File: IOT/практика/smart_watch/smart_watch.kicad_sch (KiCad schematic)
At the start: 28 parts, among them J1 Conn_01x02_Pin, J2 USB_C_Receptacle_USB2.0_16P, SW3 SW_Push, U3 KXTJ3-1057, U4 MAX30102, U5 TPS61230DRC, U6 BQ24090DGQ, U7 ESP32-WROOM-32

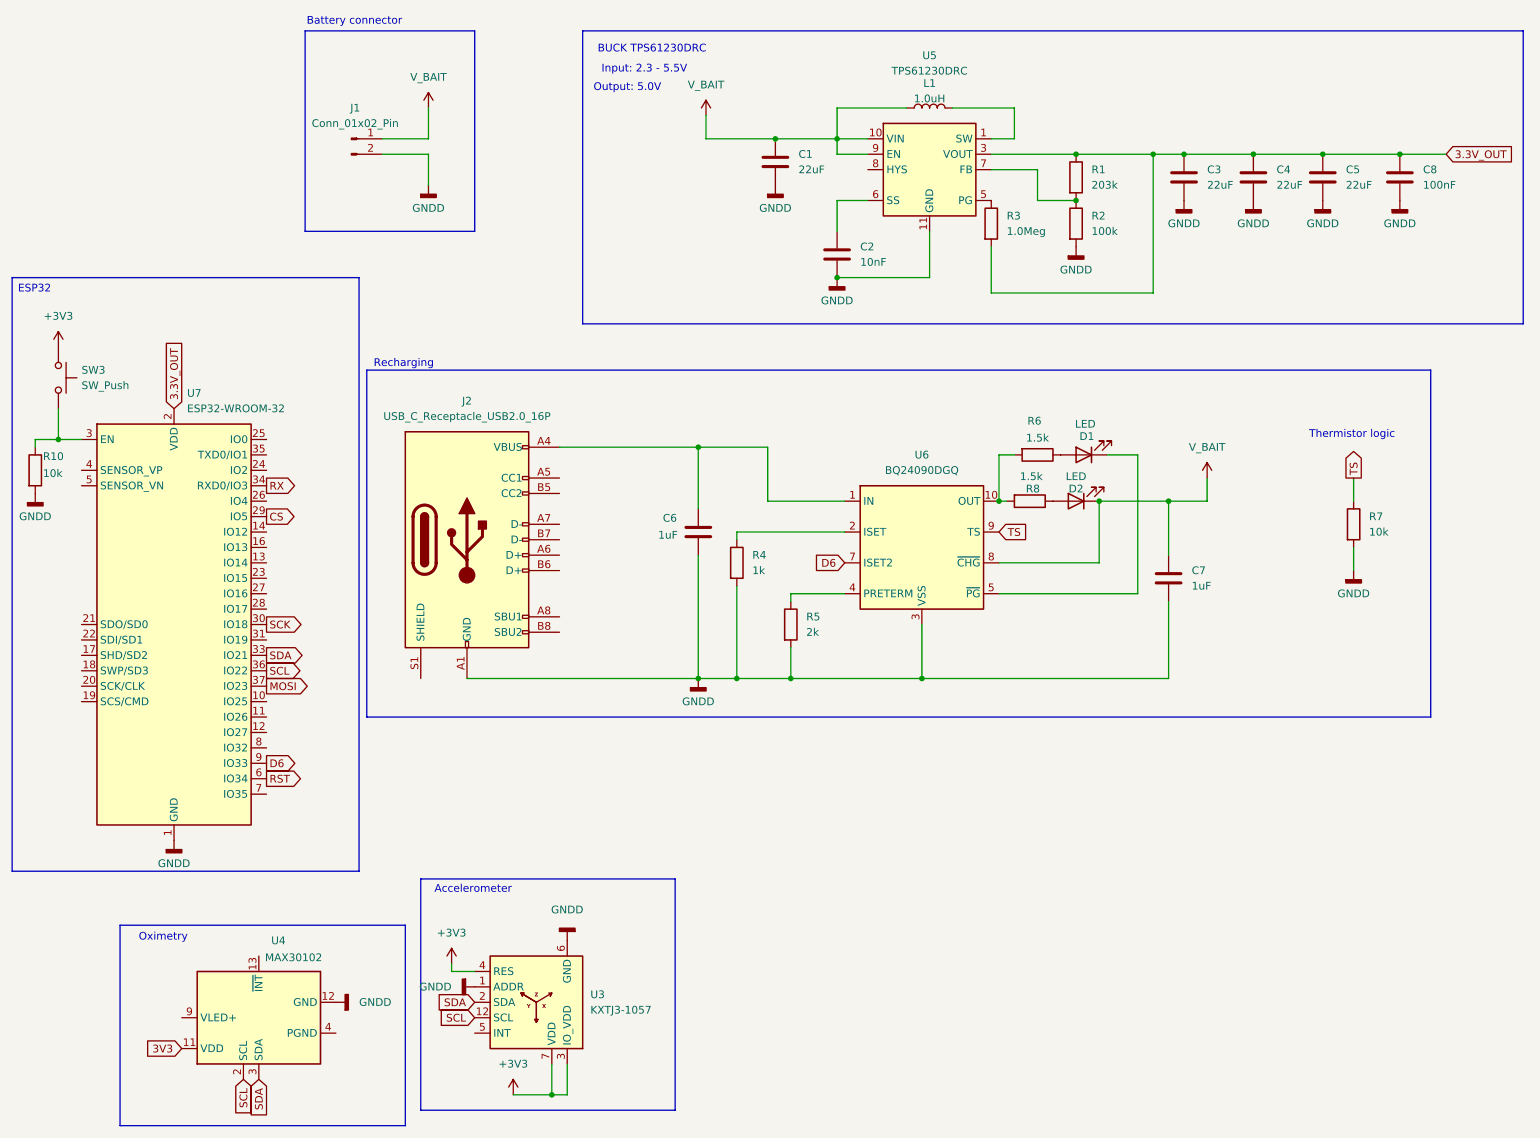
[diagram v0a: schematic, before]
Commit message: feat: adding things
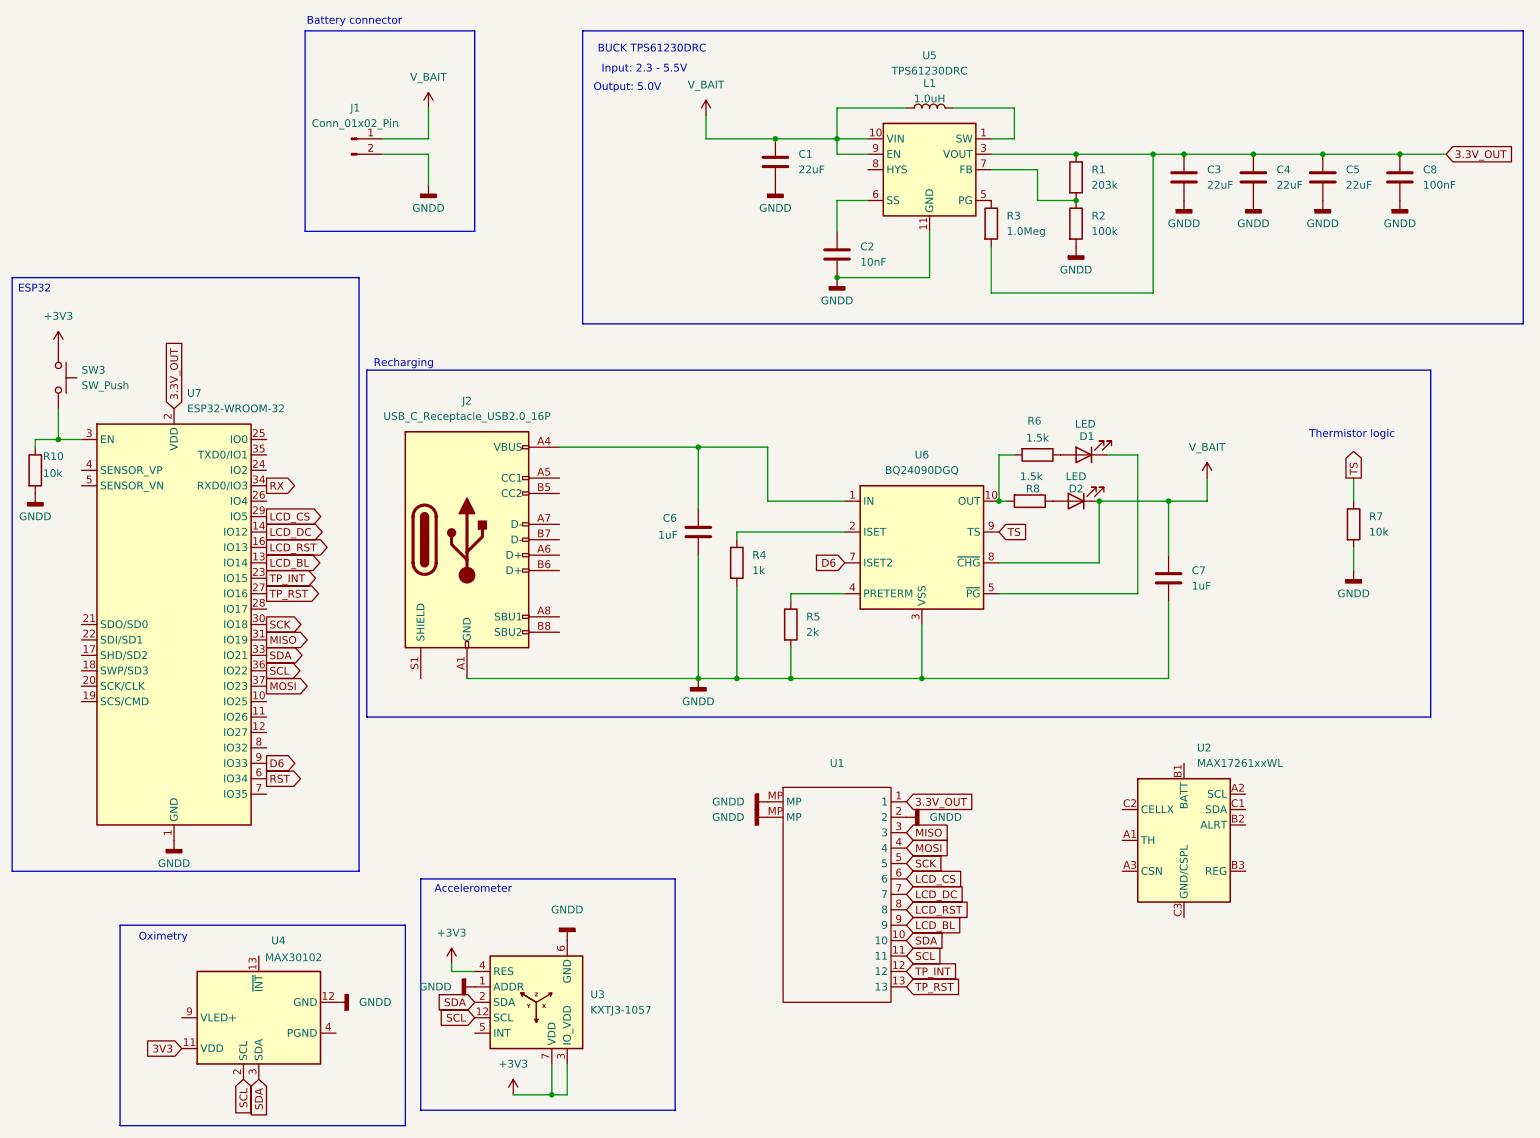
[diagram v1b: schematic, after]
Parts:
- added U1: ~, Connector_FFC:Hirose_FH12-13S-0.5SH_1x13-1MP_P0.50mm_Horizontal, symbol FH12-13S-0.5SH(55):FH12-13S-0.5SH(55)
- added U2: MAX17261xxWL, Package_BGA:Maxim_WLP-9_1.595x1.415_Layout3x3_P0.4mm_Ball0.27mm_Pad0.25mm_NSMD, symbol Battery_Management:MAX17261xxWL
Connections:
- net 3.3V_OUT: now also U1.1
- net GNDD: now also U1.2, U1.MP
- net MOSI: now also U1.4
- net SCK: now also U1.5
- net SCL: now also U1.11
- net SDA: now also U1.10
- net LCD_BL: now reaches U7.13 (IO14)
- net LCD_BL: now also U1.9
- net LCD_DC: now reaches U7.14 (IO12)
- net LCD_DC: now also U1.7
- net LCD_RST: now reaches U7.16 (IO13)
- net LCD_RST: now also U1.8
- net TP_INT: now reaches U7.23 (IO15)
- net TP_INT: now also U1.12
- net TP_RST: now reaches U7.27 (IO16)
- net TP_RST: now also U1.13
- net MISO: now reaches U7.31 (IO19)
- net MISO: now also U1.3
- net CS renamed LCD_CS
- net LCD_CS: now also U1.6
